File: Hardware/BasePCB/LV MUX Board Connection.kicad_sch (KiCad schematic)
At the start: 18 parts, among them J6 52465-2470, J9 Conn_01x02, Q1 SQJQ140E-T1_GE3, Q2 SQJQ140E-T1_GE3, Q3 SQJQ140E-T1_GE3, Q4 SQJQ140E-T1_GE3

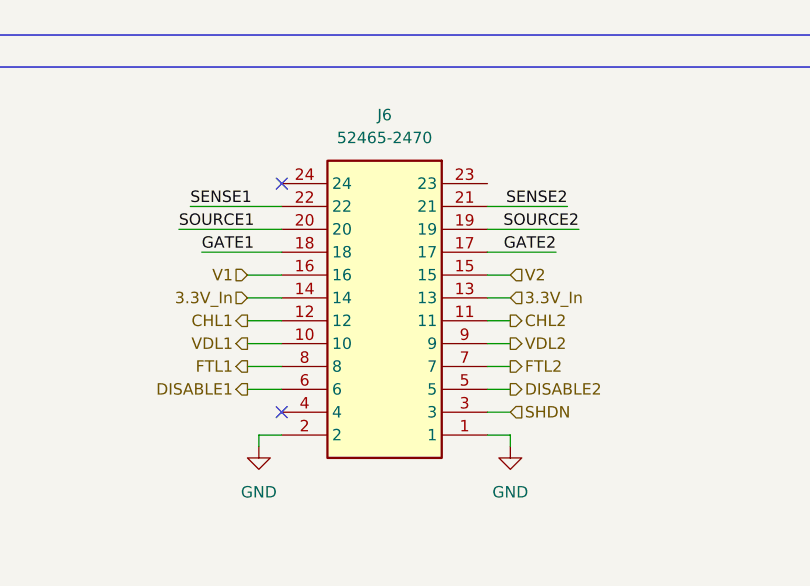
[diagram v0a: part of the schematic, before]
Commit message: talha is homiesexual
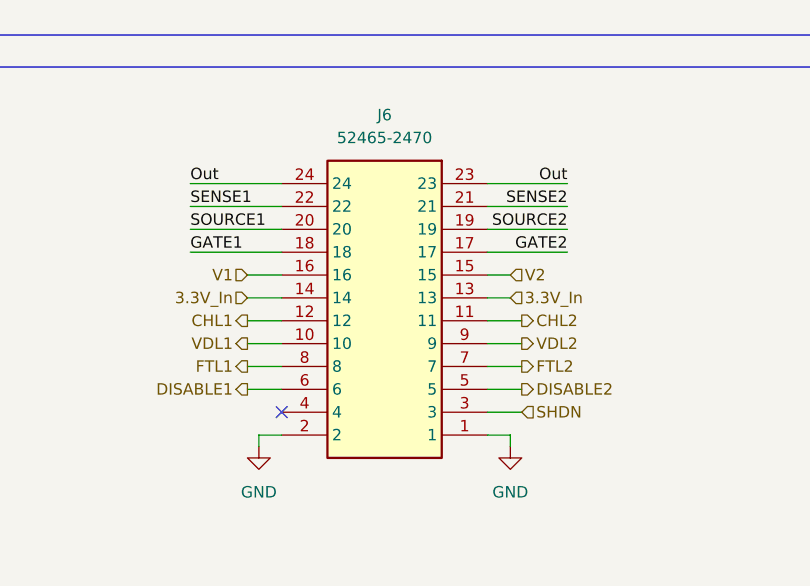
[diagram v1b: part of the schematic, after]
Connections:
- net Out: now also J6.23, J6.24
- no-connect marks 2 -> 1
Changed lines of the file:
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@@
 		(at 53.34 110.49)
 	)
-	(no_connect
-		(at 53.34 85.09)
-	)
 	(wire
 		(pts
@@
 	(wire
 		(pts
-			(xy 76.2 107.95) (xy 78.74 107.95)
+			(xy 76.2 107.95) (xy 80.01 107.95)
+		)
+		(stroke
+			(width 0)
+			(type default)
+		)
+	)
+	(wire
+		(pts
+			(xy 85.09 85.09) (xy 76.2 85.09)
 		)
 		(stroke
@@
 	(wire
 		(pts
-			(xy 76.2 105.41) (xy 78.74 105.41)
+			(xy 76.2 105.41) (xy 80.01 105.41)
 		)
 		(stroke
@@
 	(wire
 		(pts
+			(xy 43.18 85.09) (xy 53.34 85.09)
+		)
+		(stroke
+			(width 0)
+			(type default)
+		)
+	)
+	(wire
+		(pts
 			(xy 138.43 81.28) (xy 138.43 83.82)
 		)
@@
 	(wire
 		(pts
-			(xy 44.45 92.71) (xy 53.34 92.71)
+			(xy 43.18 92.71) (xy 53.34 92.71)
 		)
 		(stroke
@@
 	(wire
 		(pts
-			(xy 76.2 90.17) (xy 86.36 90.17)
+			(xy 76.2 90.17) (xy 85.09 90.17)
 		)
 		(stroke
@@
 	(wire
 		(pts
-			(xy 76.2 100.33) (xy 78.74 100.33)
-		)
-		(stroke
-			(width 0)
-			(type default)
-		)
-	)
-	(wire
-		(pts
-			(xy 41.91 90.17) (xy 53.34 90.17)
+			(xy 76.2 100.33) (xy 80.01 100.33)
+		)
+		(stroke
+			(width 0)
+			(type default)
+		)
+	)
+	(wire
+		(pts
+			(xy 43.18 90.17) (xy 53.34 90.17)
 		)
 		(stroke
@@
 	(wire
 		(pts
-			(xy 76.2 92.71) (xy 83.82 92.71)
-		)
-		(stroke
-			(width 0)
-			(type default)
-		)
-	)
-	(wire
-		(pts
-			(xy 76.2 110.49) (xy 78.74 110.49)
+			(xy 76.2 92.71) (xy 85.09 92.71)
+		)
+		(stroke
+			(width 0)
+			(type default)
+		)
+	)
+	(wire
+		(pts
+			(xy 76.2 110.49) (xy 80.01 110.49)
 		)
 		(stroke
@@
 	(wire
 		(pts
-			(xy 76.2 102.87) (xy 78.74 102.87)
+			(xy 76.2 102.87) (xy 80.01 102.87)
 		)
 		(stroke
@@
 	)
 	(label "SOURCE1"
-		(at 41.91 90.17 0)
+		(at 43.18 90.17 0)
 		(effects
 			(font
@@
 		)
 	)
+	(label "Out"
+		(at 43.18 85.09 0)
+		(effects
+			(font
+				(size 1.27 1.27)
+			)
+			(justify left bottom)
+		)
+	)
 	(label "GATE1"
 		(at 118.11 55.88 0)
@@
 	)
 	(label "GATE2"
-		(at 83.82 92.71 180)
+		(at 85.09 92.71 180)
 		(effects
 			(font
@@
 	)
 	(label "GATE1"
-		(at 44.45 92.71 0)
+		(at 43.18 92.71 0)
 		(effects
 			(font
@@
 	)
 	(label "SOURCE2"
-		(at 86.36 90.17 180)
+		(at 85.09 90.17 180)
 		(effects
 			(font
@@
 			)
 			(justify left bottom)
+		)
+	)
+	(label "Out"
+		(at 85.09 85.09 180)
+		(effects
+			(font
+				(size 1.27 1.27)
+			)
+			(justify right bottom)
 		)
 	)
@@
 	(hierarchical_label "FTL2"
 		(shape output)
-		(at 78.74 105.41 0)
+		(at 80.01 105.41 0)
 		(effects
 			(font
@@
 	(hierarchical_label "CHL2"
 		(shape output)
-		(at 78.74 100.33 0)
+		(at 80.01 100.33 0)
 		(effects
 			(font
@@
 	(hierarchical_label "VDL2"
 		(shape output)
-		(at 78.74 102.87 0)
+		(at 80.01 102.87 0)
 		(effects
 			(font
@@
 	(hierarchical_label "SHDN"
 		(shape input)
-		(at 78.74 110.49 0)
+		(at 80.01 110.49 0)
 		(effects
 			(font
@@
 	(hierarchical_label "DISABLE2"
 		(shape output)
-		(at 78.74 107.95 0)
-		(effects
-			(font
+		(at 80.01 107.95 0)
+		(effects
+			(font

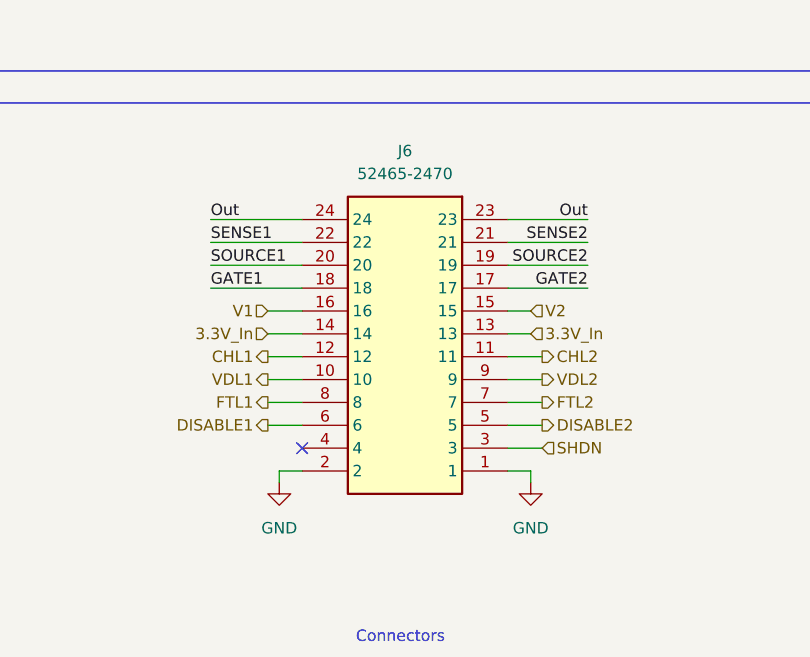
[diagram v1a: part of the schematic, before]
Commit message: Changes
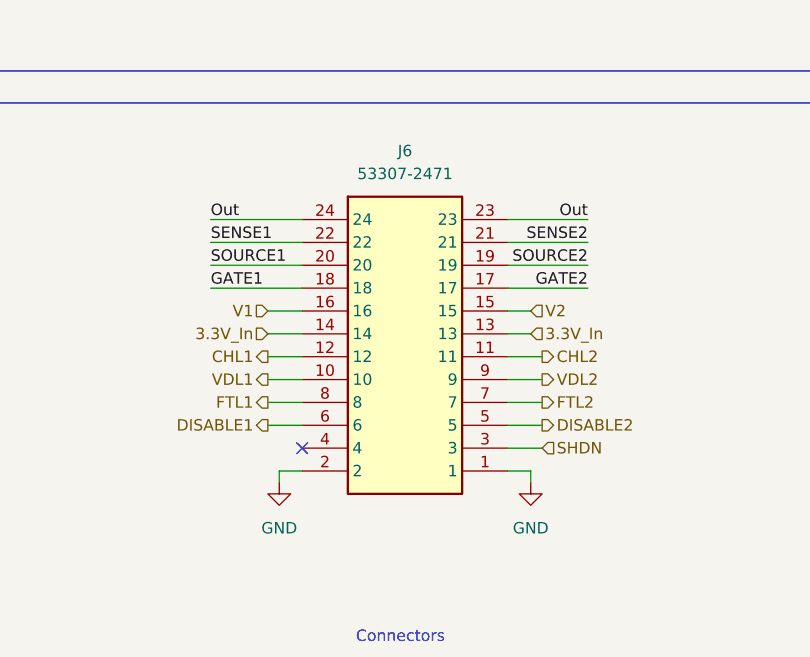
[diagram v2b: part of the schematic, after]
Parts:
- removed J6: 52465-2470, UTSVT_Connectors:524652470, symbol utsvt_connectors:52465-2470
- added J6: 53307-2471, UTSVT_Connectors:533072471, symbol utsvt_connectors:53307-2471
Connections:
- net 3.3V_In: now also J6.13, J6.14
- net CHL1: now also J6.12
- net CHL2: now also J6.11
- net DISABLE1: now also J6.6
- net DISABLE2: now also J6.5
- net FTL1: now also J6.8
- net FTL2: now also J6.7
- net GATE1: now also J6.18
- net GATE2: now also J6.17
- net GND: now also J6.1, J6.2
- net Out: now also J6.23, J6.24
- net SENSE1: now also J6.22
- net SENSE2: now also J6.21
- net SHDN: now also J6.3
- net SOURCE1: now also J6.20
- net SOURCE2: now also J6.19
- net V1: now also J6.16
- net V2: now also J6.15
- net VDL1: now also J6.10
- net VDL2: now also J6.9
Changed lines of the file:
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@@
+	)
+	(symbol
+		(lib_id "utsvt_connectors:53307-2471")
+		(at 53.34 85.09 0)
+		(unit 1)
+		(exclude_from_sim no)
+		(in_bom yes)
+		(on_board yes)
+		(dnp no)
+		(property "Reference" "J6"
+			(at 64.77 77.47 0)
+			(effects
+				(font
+					(size 1.27 1.27)
+				)
+			)
+		)
+		(property "Value" "53307-2471"
+			(at 64.77 80.01 0)
+			(effects
+				(font
+					(size 1.27 1.27)
+				)
+			)
+		)
+		(property "Footprint" "UTSVT_Connectors:533072471"
+			(at 72.39 180.01 0)
+			(effects
+				(font
+					(size 1.27 1.27)
+				)
+				(justify left top)
+				(hide yes)
+			)
+		)
+		(property "Datasheet" "https://www.mouser.com/ProductDetail/Molex/53307-2471?qs=3DzawVMofg%252Bx9c%2FNm7UacA%3D%3D&srsltid=AfmBOoo3FTqnn7XO26oYn_ClMzJiJKKwJ7tetIIyKygtiKxENiX6ckUY"
+			(at 72.39 280.01 0)
+			(effects
+				(font
+					(size 1.27 1.27)
+				)
+				(justify left top)
+				(hide yes)
+			)
+		)
+		(property "Description" "Board to Board & Mezzanine Connectors 0.8 BtB WaferAssy ST SMT 24Ckt EmbsTpPkg"
+			(at 53.34 85.09 0)
+			(effects
+				(font
+					(size 1.27 1.27)
+				)
+				(hide yes)
+			)
+		)
+		(property "P/N" "53307-2471"
+			(at 72.39 880.01 0)
+			(effects
+				(font
+					(size 1.27 1.27)
+				)
+				(justify left top)
+				(hide yes)
+			)
+		)
+		(property "Height" "3.85"
+			(at 72.39 480.01 0)
+			(effects
+				(font
+					(size 1.27 1.27)
+				)
+				(justify left top)
+				(hide yes)
+			)
+		)
+		(property "Mouser Part Number" "538-53307-2471"
+			(at 72.39 580.01 0)
+			(effects
+				(font
+					(size 1.27 1.27)
+				)
+				(justify left top)
+				(hide yes)
+			)
+		)
+		(property "Mouser Price/Stock" "https://www.mouser.co.uk/ProductDetail/Molex/53307-2471?qs=3DzawVMofg%252Bx9c%2FNm7UacA%3D%3D"
+			(at 72.39 680.01 0)
+			(effects
+				(font
+					(size 1.27 1.27)
+				)
+				(justify left top)
+				(hide yes)
+			)
+		)
+		(pin "20"
+		)
+		(pin "22"
+		)
+		(pin "10"
+		)
+		(pin "6"
+		)
+		(pin "4"
+		)
+		(pin "23"
+		)
+		(pin "19"
+		)
+		(pin "16"
+		)
+		(pin "12"
+		)
+		(pin "24"
+		)
+		(pin "14"
+		)
+		(pin "18"
+		)
+		(pin "8"
+		)
+		(pin "2"
+		)
+		(pin "21"
+		)
+		(pin "3"
+		)
+		(pin "11"
+		)
+		(pin "7"
+		)
+		(pin "5"
+		)
+		(pin "13"
+		)
+		(pin "15"
+		)
+		(pin "1"
+		)
+		(pin "9"
+		)
+		(pin "17"
+		)
+		(instances
+			(project "LV Carrier Board"
+				(path "/c5c5922b-1600-4b67-acf3-33264cecd75b/674ca403-ac68-42d3-a671-b4e759ecad50"
+					(reference "J6")
+					(unit 1)
+				)
+			)
+		)
 	)
 	(symbol
@@
 					(unit 1)
 				)
-			)
-		)
-	)
-	(symbol
-		(lib_id "utsvt_connectors:52465-2470")
-		(at 76.2 85.09 0)
-		(mirror y)
-		(unit 1)
-		(exclude_from_sim no)
-		(in_bom yes)
-		(on_board yes)
-		(dnp no)
-		(property "Reference" "J6"
-			(at 64.77 77.47 0)
-			(effects
-				(font
-					(size 1.27 1.27)
-				)
-			)
-		)
-		(property "Value" "52465-2470"
-			(at 64.77 80.01 0)
-			(effects
-				(font
-					(size 1.27 1.27)
-				)
-			)
-		)
-		(property "Footprint" "UTSVT_Connectors:524652470"
-			(at 57.15 180.01 0)
-			(effects
-				(font
-					(size 1.27 1.27)
-				)
-				(justify left top)
-				(hide yes)
-			)
-		)
-		(property "Datasheet" "https://www.molex.com/pdm_docs/sd/524652470_sd.pdf"
-			(at 57.15 280.01 0)
-			(effects
-				(font
-					(size 1.27 1.27)
-				)
-				(justify left top)
-				(hide yes)
-			)
-		)
-		(property "Description" "24 pin board-board connector"
-			(at 92.202 81.28 0)
-			(effects
-				(font
-					(size 1.27 1.27)
-				)
-				(hide yes)
-			)
-		)
-		(property "Height" "3.55"
-			(at 57.15 480.01 0)
-			(effects
-				(font
-					(size 1.27 1.27)
-				)
-				(justify left top)
-				(hide yes)
-			)
-		)
-		(property "Mouser Part Number" "538-52465-2470"
-			(at 57.15 580.01 0)
-			(effects
-				(font
-					(size 1.27 1.27)
-				)
-				(justify left top)
-				(hide yes)
-			)
-		)
-		(property "Mouser Price/Stock" "https://www.mouser.co.uk/ProductDetail/Molex/52465-2470?qs=sEN%2FkO1EG6Yhu4DkZwbE7Q%3D%3D"
-			(at 57.15 680.01 0)
-			(effects
-				(font
-					(size 1.27 1.27)
-				)
-				(justify left top)
-				(hide yes)
-			)
-		)
-		(property "Manufacturer_Name" "Molex"
-			(at 57.15 780.01 0)
-			(effects
-				(font
-					(size 1.27 1.27)
-				)
-				(justify left top)
-				(hide yes)
-			)
-		)
-		(property "P/N" "52465-2470"
-			(at 57.15 880.01 0)
-			(effects
-				(font
-					(size 1.27 1.27)
-				)
-				(justify left top)
-				(hide yes)
-			)
-		)
-		(pin "6"
-		)
-		(pin "24"
-		)
-		(pin "19"
-		)
-		(pin "23"
-		)
-		(pin "15"
-		)
-		(pin "9"
-		)
-		(pin "21"
-		)
-		(pin "3"
-		)
-		(pin "22"
-		)
-		(pin "18"
-		)
-		(pin "8"
-		)
-		(pin "20"
-		)
-		(pin "11"
-		)
-		(pin "7"
-		)
-		(pin "1"
-		)
-		(pin "5"
-		)
-		(pin "10"
-		)
-		(pin "14"
-		)
-		(pin "17"
-		)
-		(pin "16"
-		)
-		(pin "13"
-		)
-		(pin "12"
-		)
-		(pin "2"
-		)
-		(pin "4"
-		)
-		(instances
-			(project "LV Carrier Board"
-				(path "/c5c5922b-1600-4b67-acf3-33264cecd75b/674ca403-ac68-42d3-a671-b4e759ecad50"
-					(reference "J6")
-					(unit 1)
-				)

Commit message: Changes
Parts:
- C1, C2, CMOSFET1, CMOSFET3: footprint Capacitor_SMD:C_0805_2012Metric -> Capacitor_SMD:C_0603_1608Metric
- R3, R4: footprint Resistor_SMD:R_0805_2012Metric -> Resistor_SMD:R_0603_1608Metric
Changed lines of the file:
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@@
 			)
 		)
-		(property "Footprint" "Resistor_SMD:R_0805_2012Metric"
+		(property "Footprint" "Resistor_SMD:R_0603_1608Metric"
 			(at 211.328 35.56 90)
 			(effects
@@
 			)
 		)
-		(property "Footprint" "Capacitor_SMD:C_0805_2012Metric"
+		(property "Footprint" "Capacitor_SMD:C_0603_1608Metric"
 			(at 208.5848 46.99 0)
 			(effects
@@
 			)
 		)
-		(property "Footprint" "Capacitor_SMD:C_0805_2012Metric"
+		(property "Footprint" "Capacitor_SMD:C_0603_1608Metric"
 			(at 60.6552 48.26 0)
 			(effects
@@
 			)
 		)
-		(property "Footprint" "Capacitor_SMD:C_0805_2012Metric"
+		(property "Footprint" "Capacitor_SMD:C_0603_1608Metric"
 			(at 88.9 37.7952 0)
 			(effects
@@
 			)
 		)
-		(property "Footprint" "Capacitor_SMD:C_0805_2012Metric"
+		(property "Footprint" "Capacitor_SMD:C_0603_1608Metric"
 			(at 180.34 37.7952 0)
 			(effects
@@
 			)
 		)
-		(property "Footprint" "Resistor_SMD:R_0805_2012Metric"
+		(property "Footprint" "Resistor_SMD:R_0603_1608Metric"
 			(at 57.912 36.83 90)
 			(effects

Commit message: ts not performative
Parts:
- J6: footprint UTSVT_Connectors:533072471 -> LV Carrier Library:LVMux
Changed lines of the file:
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@@
 			)
 		)
-		(property "Footprint" "UTSVT_Connectors:533072471"
+		(property "Footprint" "LV Carrier Library:LVMux"
 			(at 72.39 180.01 0)
 			(effects

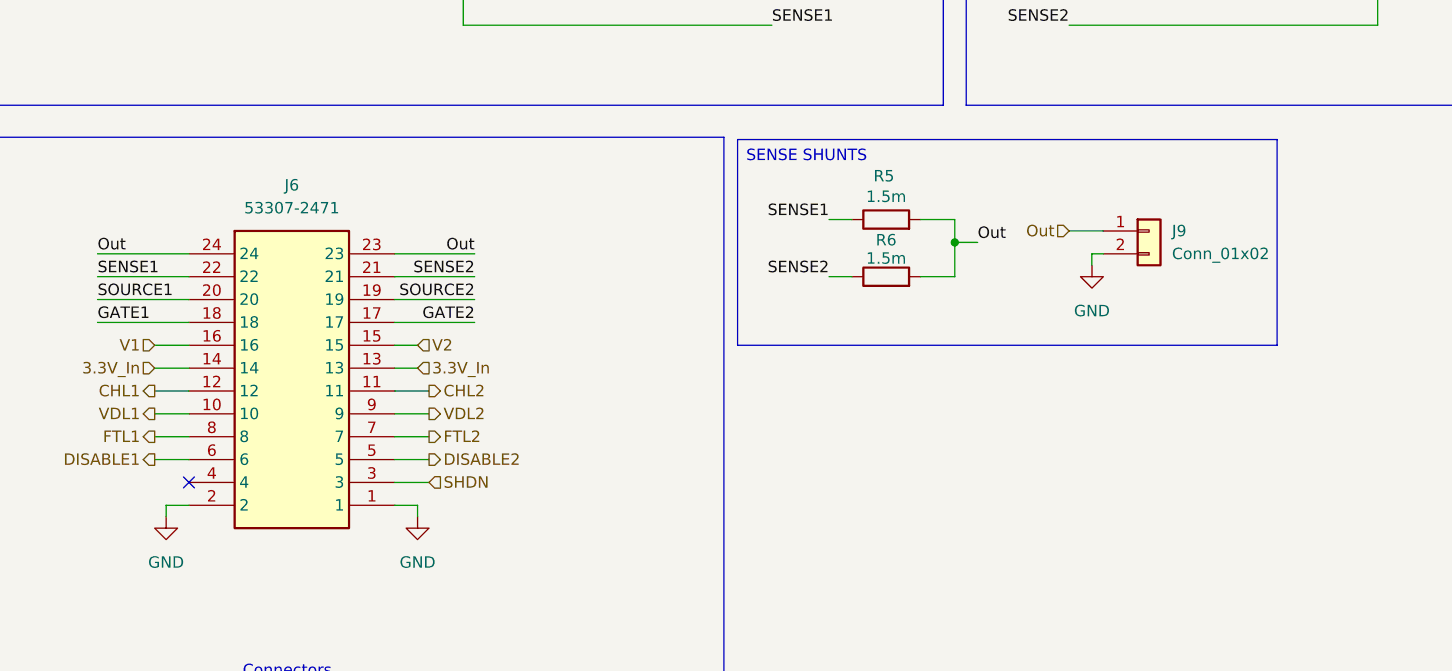
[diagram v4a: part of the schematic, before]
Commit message: lakshay and changxu bullied me incessantly for hours
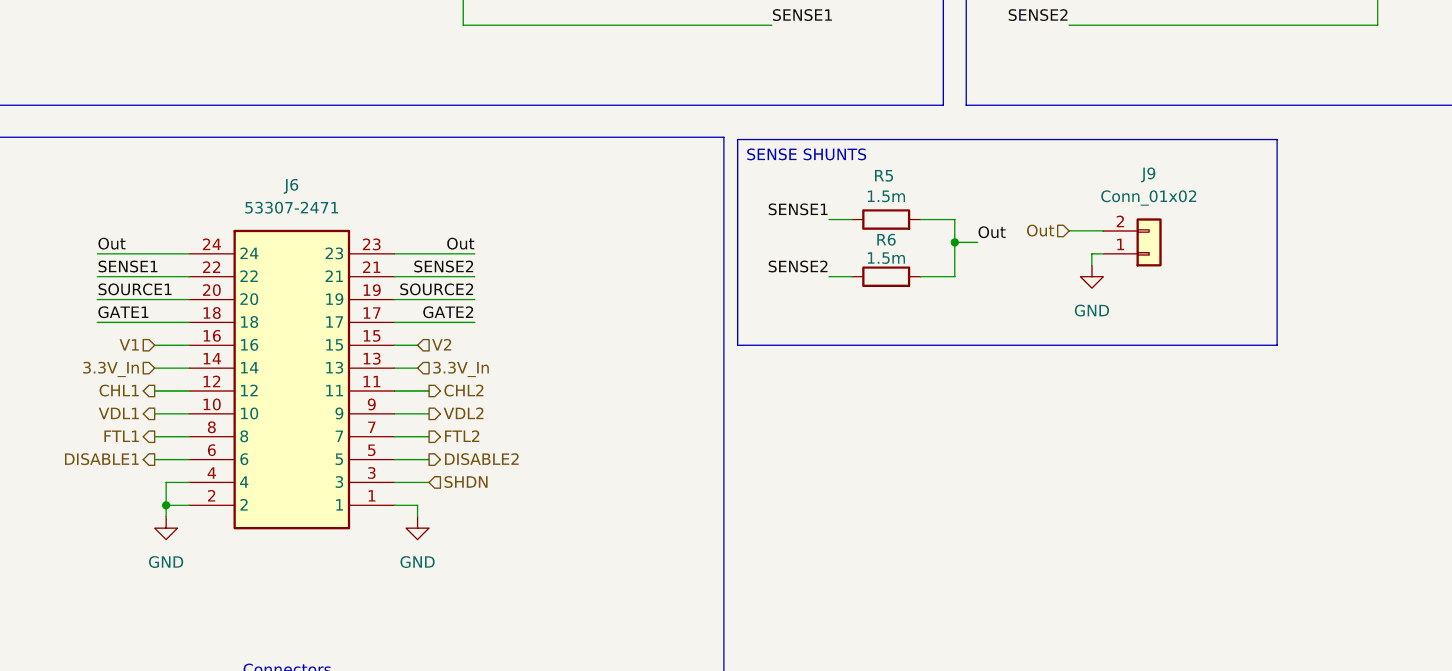
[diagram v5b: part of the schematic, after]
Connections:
- net GND: now also J6.4, J9.1 (Pin_1); no longer J9.2 (Pin_2)
- net Out: now also J9.2 (Pin_2); no longer J9.1 (Pin_1)
- no-connect marks 1 -> 0
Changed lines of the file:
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@@
+	)
+	(junction
+		(at 50.8 113.03)
+		(diameter 0)
+		(color 0 0 0 0)
 	)
 	(junction
@@
 		(color 0 0 0 0)
 	)
-	(no_connect
-		(at 53.34 110.49)
-	)
 	(wire
 		(pts
@@
 	(wire
 		(pts
+			(xy 53.34 110.49) (xy 50.8 110.49)
+		)
+		(stroke
+			(width 0)
+			(type default)
+		)
+	)
+	(wire
+		(pts
 			(xy 43.18 85.09) (xy 53.34 85.09)
 		)
@@
 		(pts
 			(xy 151.13 82.55) (xy 154.94 82.55)
+		)
+		(stroke
+			(width 0)
+			(type default)
+		)
+	)
+	(wire
+		(pts
+			(xy 50.8 110.49) (xy 50.8 113.03)
 		)
 		(stroke
@@
 	(symbol
 		(lib_id "Connector_Generic:Conn_01x02")
-		(at 160.02 82.55 0)
+		(at 160.02 85.09 0)
+		(mirror x)
 		(unit 1)
 		(exclude_from_sim no)
@@
 		(on_board yes)
 		(dnp no)
-		(fields_autoplaced yes)
 		(property "Reference" "J9"
-			(at 162.56 82.5499 0)
-			(effects
-				(font
-					(size 1.27 1.27)
-				)
-				(justify left)
+			(at 160.02 76.2 0)
+			(effects
+				(font
+					(size 1.27 1.27)
+				)
 			)
 		)
 		(property "Value" "Conn_01x02"
-			(at 162.56 85.0899 0)
-			(effects
-				(font
-					(size 1.27 1.27)
-				)
-				(justify left)
+			(at 160.02 78.74 0)
+			(effects
+				(font
+					(size 1.27 1.27)
+				)
 			)
 		)
 		(property "Footprint" "LV Carrier Library:AMASS_XT30UPB-M_1x02_P5.0mm_Vertical"
-			(at 160.02 82.55 0)
+			(at 160.02 85.09 0)
 			(effects
 				(font
@@
 		)
 		(property "Datasheet" "~"
-			(at 160.02 82.55 0)
+			(at 160.02 85.09 0)
 			(effects
 				(font
@@
 		)
 		(property "Description" "Generic connector, single row, 01x02, script generated (kicad-library-utils/schlib/autogen/connector/)"
-			(at 160.02 82.55 0)
-			(effects
-				(font
+			(at 160.02 85.09 0)
+			(effects
+				(font
